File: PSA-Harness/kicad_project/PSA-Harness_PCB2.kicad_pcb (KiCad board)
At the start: 4 copper layers, 27.4 x 53.6 mm, 10 parts, among them J1 to_EPS_1, J2 to_EPS_2, J3 to_ESP_3, J7 USB_C_Receptacle, J8 B2B_1, J9 B2B_2, K1 G6K-2G-Y DC5

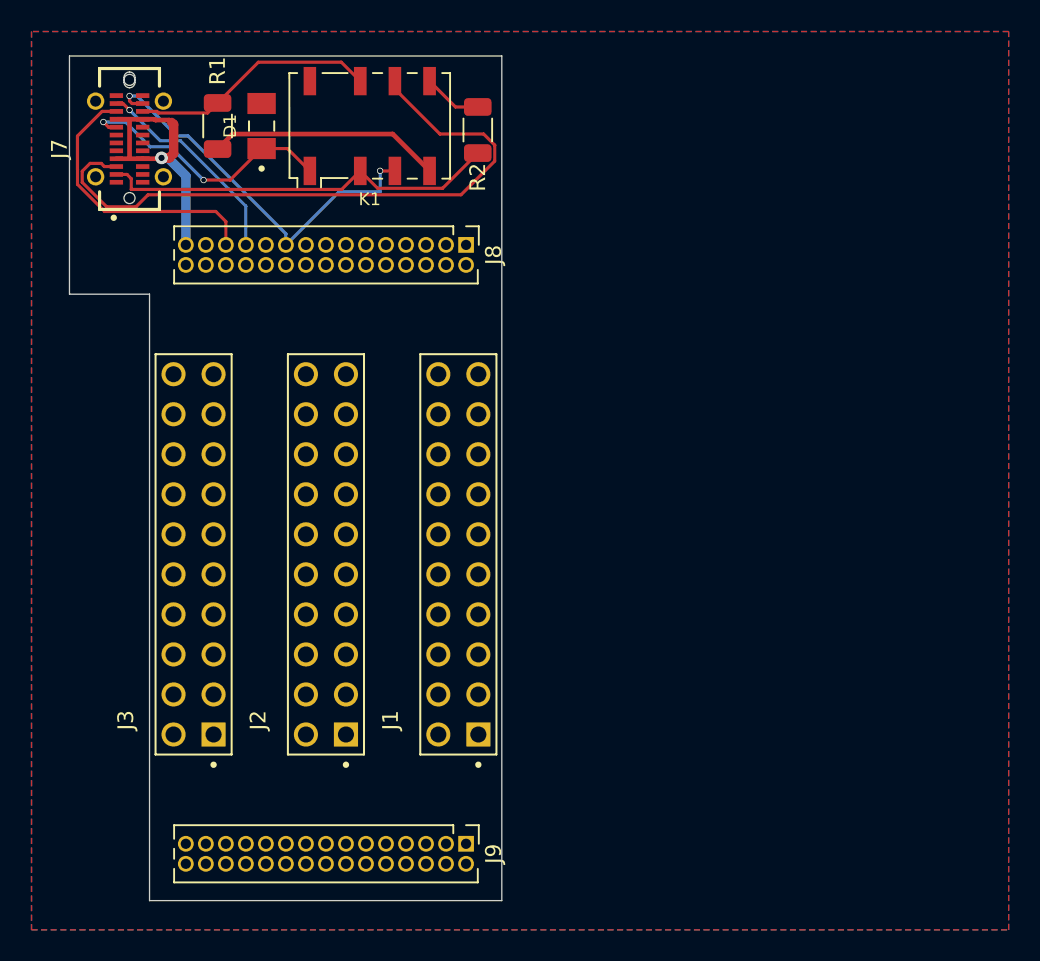
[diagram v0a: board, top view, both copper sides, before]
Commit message: PCB1+2 routed
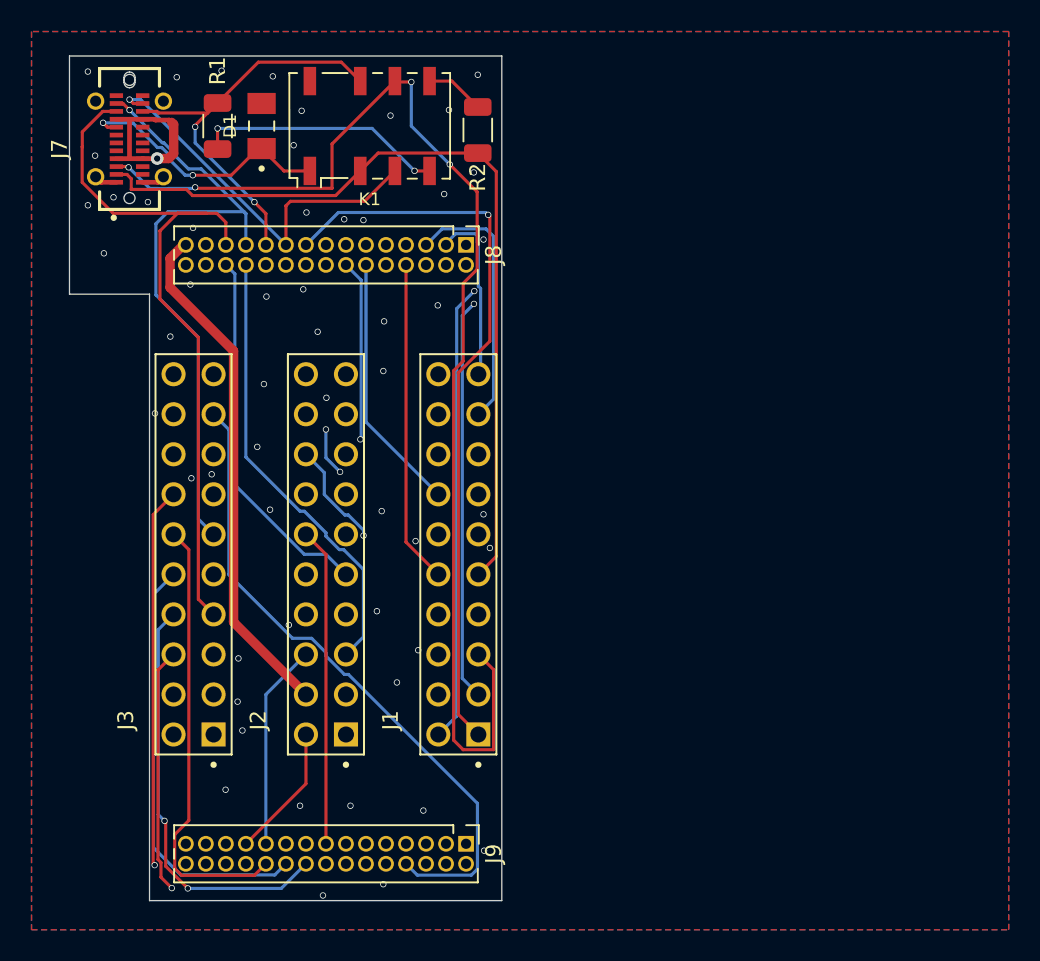
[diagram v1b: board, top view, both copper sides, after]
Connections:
- J7 pad S2: (no net) -> GND
- J7 pad S3: (no net) -> GND
- J7 pad S4: (no net) -> GND
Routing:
- net 50: track 0.00 -> 52.7 mm, vias 0 -> 4
- net 4: track 0.00 -> 49.6 mm, vias 0 -> 3
- net 1: track 0.00 -> 46.8 mm, vias 0 -> 1
- net 48: track 0.00 -> 45.0 mm, vias 0 -> 1
- net 29: track 0.00 -> 44.3 mm, vias 0 -> 1
- net 49: track 0.00 -> 41.6 mm
- net 2: track 0.00 -> 41.6 mm, vias 0 -> 1
- net 58: track 0.00 -> 36.8 mm, vias 0 -> 1
- net CAN0_L: track 40.5 -> 77.2 mm, vias 0 -> 4
- net 47: track 0.00 -> 36.6 mm
- net 28: track 0.00 -> 36.4 mm, vias 0 -> 1
- net 30: track 0.00 -> 35.9 mm, vias 0 -> 1
- net 40: track 0.00 -> 33.2 mm
- net +12V: track 18.3 -> 51.1 mm
- net 11: track 0.00 -> 32.4 mm, vias 0 -> 1
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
